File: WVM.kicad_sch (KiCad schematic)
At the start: 7 parts, among them J1 USB4215-03-A_REVA, U1 IIS3DWBTR, U2 MCP9808_DFN, U3 CH340C, U4 TPS63036YFGT, U5 NORA-W106-00B, U6 TP4056-42-ESOP8

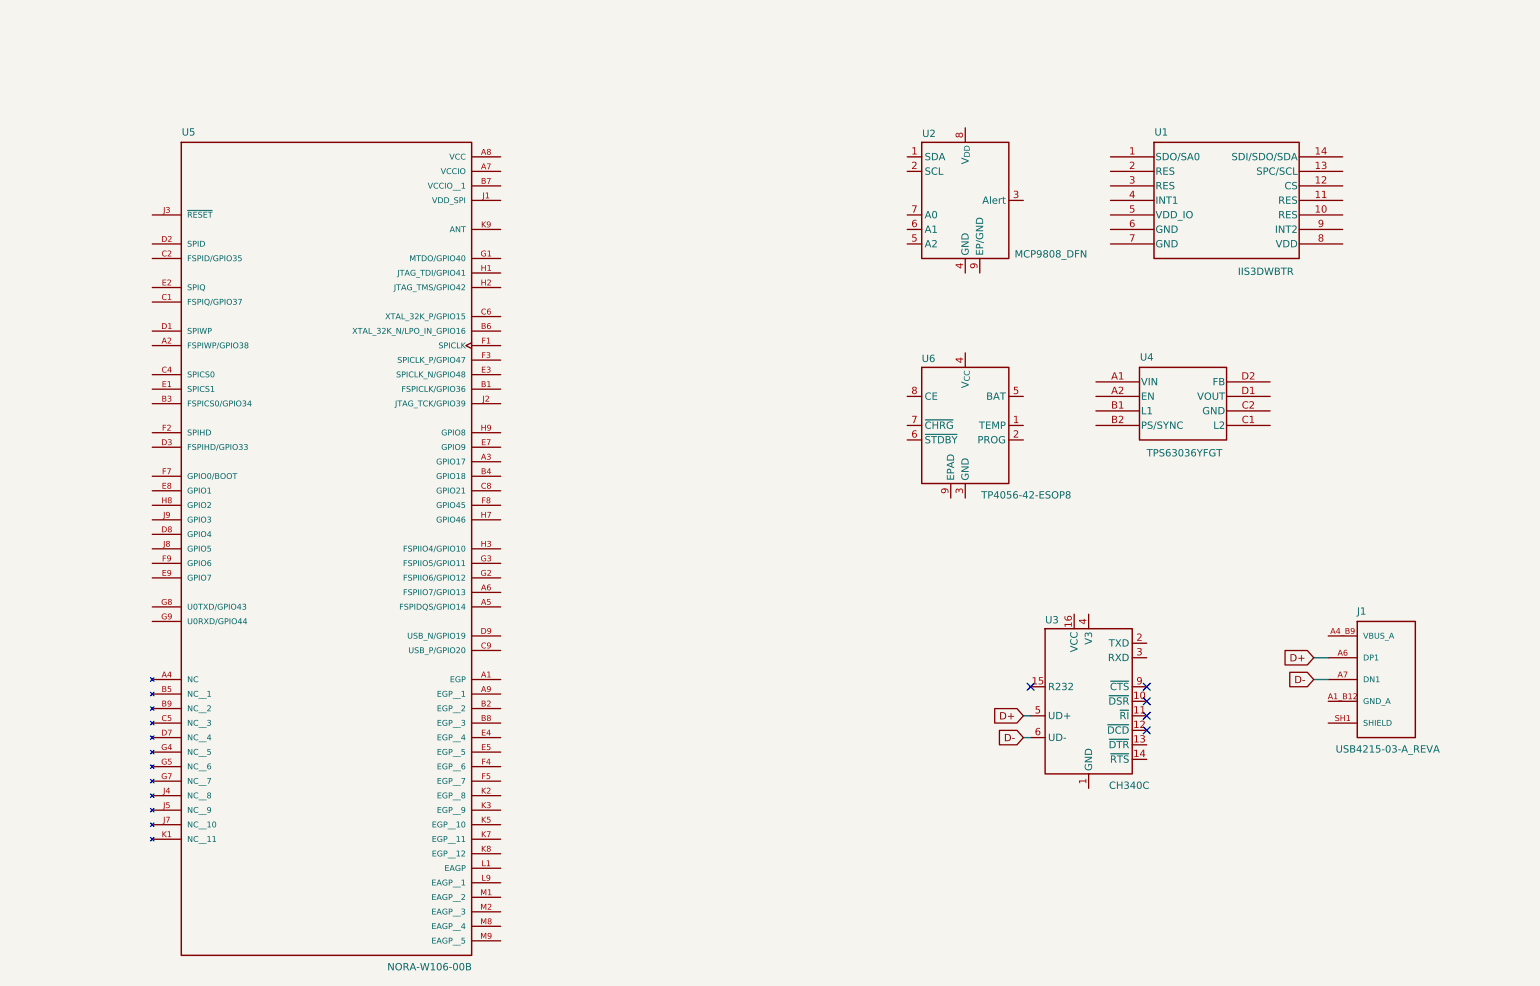
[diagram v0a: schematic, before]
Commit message: Modified Schematic 07.10.25
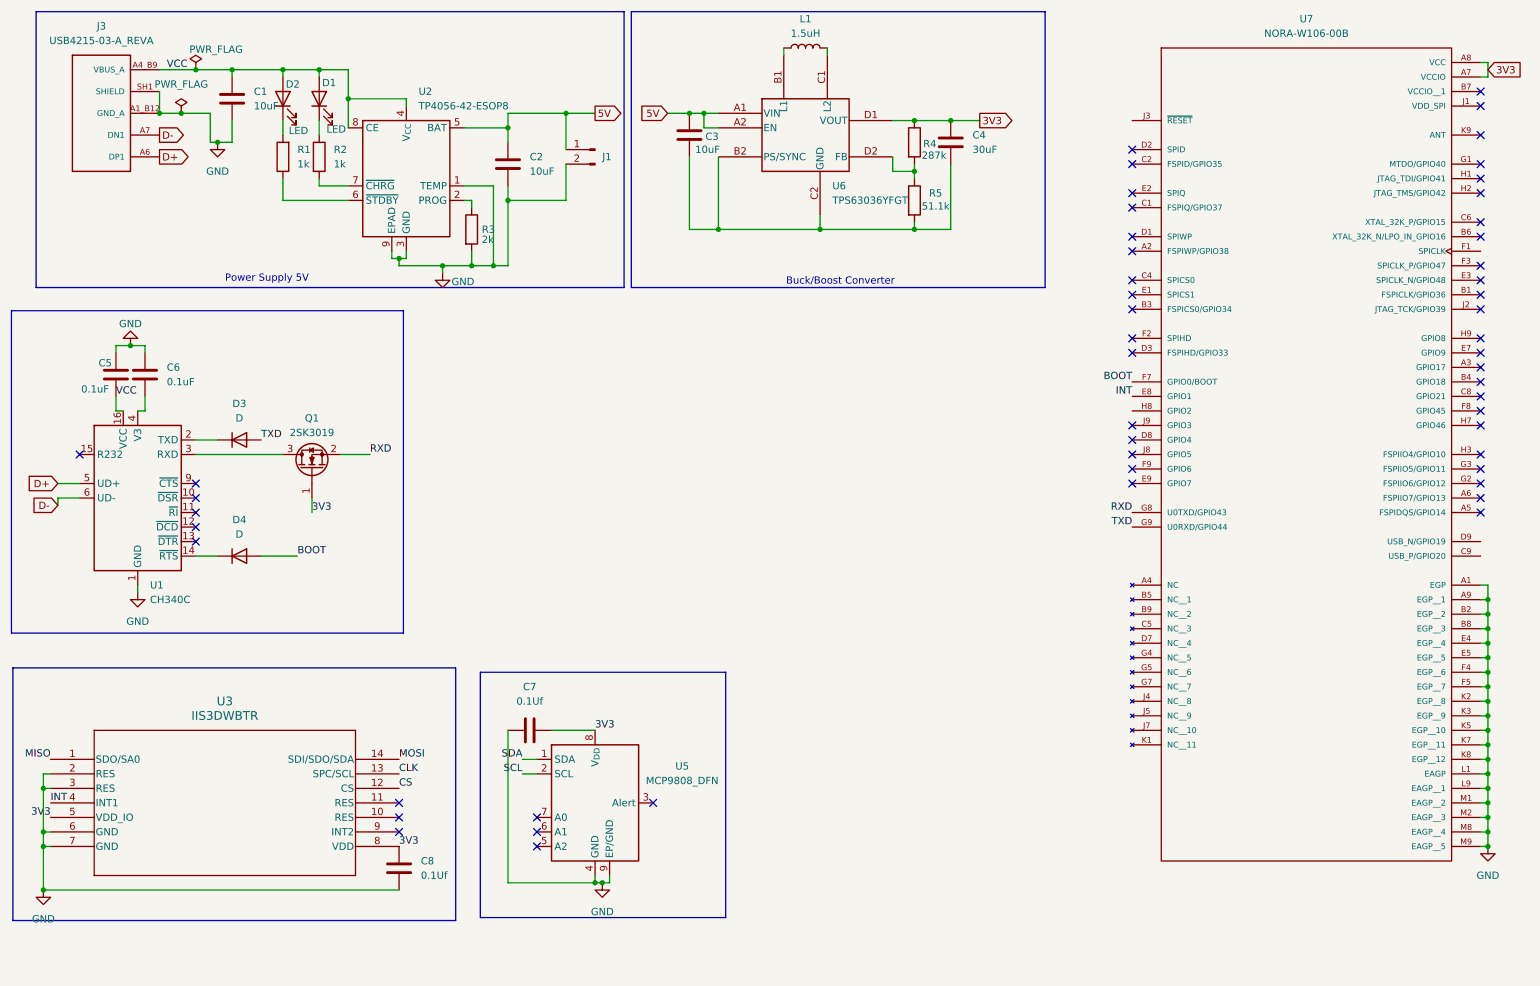
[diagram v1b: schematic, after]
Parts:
- removed J1: USB4215-03-A_REVA, USB4215-03-A:USB4215-03-A_REVA, symbol USB4215-03-A_REVA:USB4215-03-A_REVA
- removed U1: IIS3DWBTR, IIS3DWBTR:LGA-14L_2P5X3X0P83_STM, symbol IIS3DWBTR:IIS3DWBTR
- removed U2: MCP9808_DFN, Package_DFN_QFN:DFN-8-1EP_3x2mm_P0.5mm_EP1.7x1.4mm, symbol Sensor_Temperature:MCP9808_DFN
- removed U3: CH340C, Package_SO:SOIC-16_3.9x9.9mm_P1.27mm, symbol Interface_USB:CH340C
- removed U4: TPS63036YFGT, TPS63036YFGT:TPS63036YFGT, symbol TPS63036YFGT:TPS63036YFGT
- removed U5: NORA-W106-00B, NORA-W106-00B:XCVR_NORA-W106-00B, symbol NORA-W106-00B:NORA-W106-00B
- removed U6: TP4056-42-ESOP8, Package_SO:SOIC-8-1EP_3.9x4.9mm_P1.27mm_EP2.41x3.3mm_ThermalVias, symbol Battery_Management:TP4056-42-ESOP8
- added C1, C2, C3: 10uF, symbol Device:C
- added C4: 30uF, symbol Device:C
- added C5, C6: 0.1uF, symbol Device:C
- added C7, C8: 0.1Uf, symbol Device:C
- added D1, D2: LED, symbol Device:LED
- added D3, D4: D, symbol Device:D
- added J1: Conn_01x02_Pin, daFootprintsBX:JST_S2B-PH-SM4-TB, symbol Connector:Conn_01x02_Pin
- added J3: USB4215-03-A_REVA, USB4215-03-A:USB4215-03-A_REVA, symbol USB4215-03-A_REVA:USB4215-03-A_REVA
- added L1: 1.5uH, symbol Device:L
- added Q1: 2SK3019, Package_TO_SOT_SMD:SOT-523, symbol Transistor_FET:2SK3019
- added R1, R2: 1k, symbol Device:R
- added R3: 2k, symbol Device:R
- added R4: 287k, symbol Device:R
- added R5: 51.1k, symbol Device:R
- added U1: CH340C, Package_SO:SOIC-16_3.9x9.9mm_P1.27mm, symbol Interface_USB:CH340C
- added U2: TP4056-42-ESOP8, Package_SO:SOIC-8-1EP_3.9x4.9mm_P1.27mm_EP2.41x3.3mm_ThermalVias, symbol Battery_Management:TP4056-42-ESOP8
- added U3: IIS3DWBTR, LGA-14L_2P5X3X0P83_STM, symbol IIS3DWBTR:IIS3DWBTR
- added U5: MCP9808_DFN, Package_DFN_QFN:DFN-8-1EP_3x2mm_P0.5mm_EP1.7x1.4mm, symbol Sensor_Temperature:MCP9808_DFN
- added U6: TPS63036YFGT, TPS63036YFGT:TPS63036YFGT, symbol TPS63036YFGT:TPS63036YFGT
- added U7: NORA-W106-00B, NORA-W106-00B:XCVR_NORA-W106-00B, symbol NORA-W106-00B:NORA-W106-00B
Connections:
- net D+: now also J3.A6 (DP1), U1.5 (UD+)
- net D-: now also J3.A7 (DN1), U1.6 (UD-)
- new net: Q1.3 (D), U1.3 (RXD)
- new net: C3.2, C4.2, R5.2, U6.B2 (PS/SYNC), U6.C2 (GND)
- new net: R3.1, U2.2 (PROG)
- new net: R1.1, U2.6 (~{STDBY})
- new net: R2.2, U2.7 (~{CHRG})
- new net: D2.1 (K), R1.2
- new net: D4.1 (K), U1.14 (~{RTS})
- new net: C6.2, U1.4 (V3)
- new net: D3.1 (K), U1.2 (TXD)
- new net: L1.1, U6.B1 (L1)
- new net: L1.2, U6.C1 (L2)
- new net: R4.2, R5.1, U6.D2 (FB)
- new net: D1.1 (K), R2.1
- new net 3V3: C4.1, C7.2, C8.1, Q1.1 (G), R4.1, U3.5 (VDD_IO), U3.8 (VDD), U5.8 (V_{DD}), U6.D1 (VOUT), U7.A7 (VCCIO), U7.A8 (VCC)
- new net 5V: C2.1, C3.1, J1.1 (Pin_1), U2.5 (BAT), U6.A1 (VIN), U6.A2 (EN)
- new net BOOT: D4.2 (A), U7.F7 (GPIO0/BOOT)
- new net CLK: U3.13 (SPC/SCL)
- new net CS: U3.12 (CS)
- new net GND: C1.2, C2.2, C5.1, C6.1, C7.1, C8.2, J1.2 (Pin_2), J3.A1_B12 (GND_A), J3.SH1 (SHIELD), R3.2, U1.1 (GND), U2.1 (TEMP), U2.3 (GND), U2.9 (EPAD), U3.2 (RES), U3.3 (RES), U3.6 (GND), U3.7 (GND), U5.4 (GND), U5.9 (EP/GND), U7.A1 (EGP), U7.A9 (EGP__1), U7.B2 (EGP__2), U7.B8 (EGP__3), U7.E4 (EGP__4), U7.E5 (EGP__5), U7.F4 (EGP__6), U7.F5 (EGP__7), U7.K2 (EGP__8), U7.K3 (EGP__9), U7.K5 (EGP__10), U7.K7 (EGP__11), U7.K8 (EGP__12), U7.L1 (EAGP), U7.L9 (EAGP__1), U7.M1 (EAGP__2), U7.M2 (EAGP__3), U7.M8 (EAGP__4), U7.M9 (EAGP__5)
- new net INT: U3.4 (INT1), U7.E8 (GPIO1)
- new net MISO: U3.1 (SDO/SA0)
- new net MOSI: U3.14 (SDI/SDO/SDA)
- new net RXD: Q1.2 (S), U7.G8 (U0TXD/GPIO43)
- new net SCL: U5.2 (SCL)
- new net SDA: U5.1 (SDA)
- new net TXD: D3.2 (A), U7.G9 (U0RXD/GPIO44)
- new net VCC: C1.1, C5.2, D1.2 (A), D2.2 (A), J3.A4_B9 (VBUS_A), U1.16 (VCC), U2.4 (V_{CC}), U2.8 (CE)
- no-connect marks 5 -> 53
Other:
- note added: "Buck/Boost Converter"
- note added: "Power Supply 5V"
